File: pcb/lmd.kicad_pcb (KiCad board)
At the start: 2 copper layers, 22.6 x 26.5 mm, 27 parts, among them J1 Conn_01x05, J2 conn:Conn_01x04, J3 Conn_01x03, J4 Conn_01x04, J6 conn:Conn_01x04, U1 TLE493D, U2 TJA1028, U3 DRV8848, U4 PIC16(L)F15323

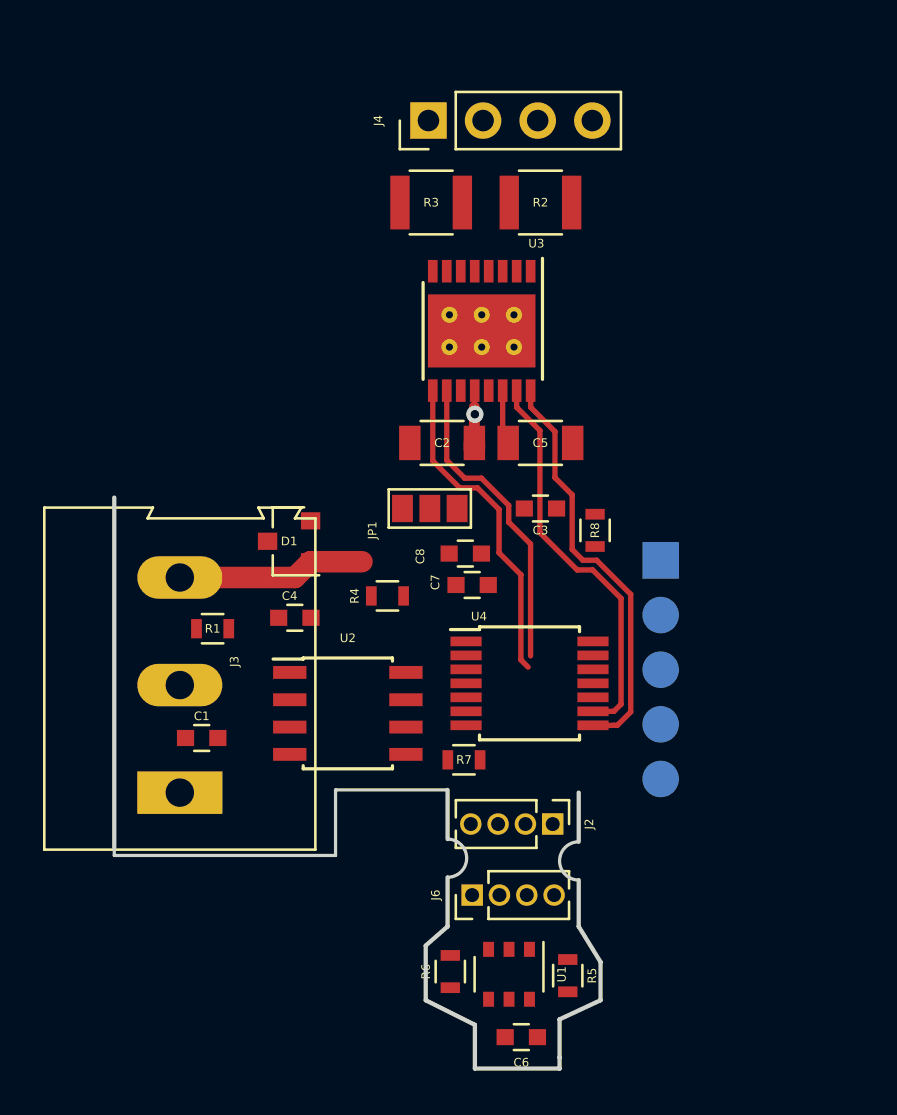
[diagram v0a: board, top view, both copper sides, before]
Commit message: Layout fix
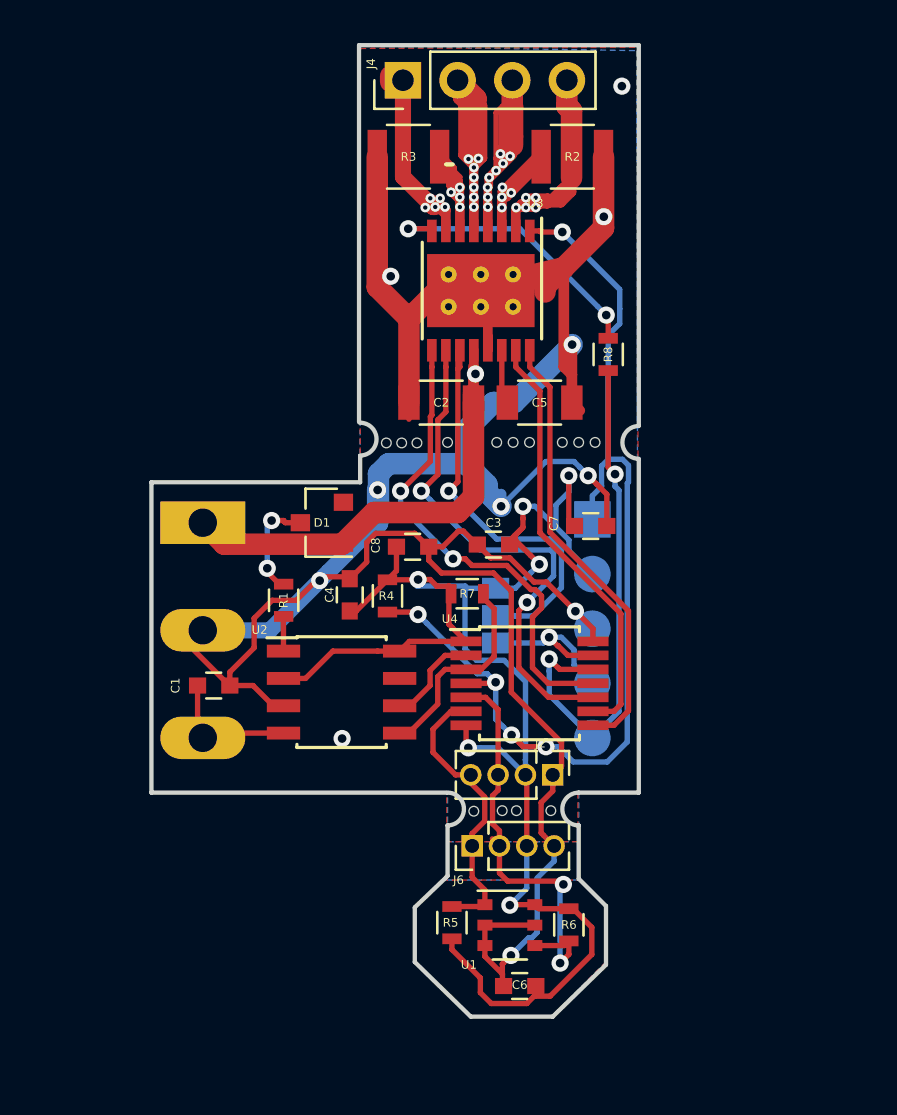
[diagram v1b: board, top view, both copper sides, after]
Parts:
- removed the J6 at (120.8, 129.2)
- added J6: Conn_01x04, ucan_custom:hole, F.Cu at (117.5, 108.2)
- added J6: Conn_01x04, ucan_custom:hole, F.Cu at (116.8, 108.2)
- added J6: Conn_01x04, ucan_custom:hole, F.Cu at (124.4, 125.3)
- added J6: Conn_01x04, ucan_custom:hole, F.Cu at (120.9, 125.3)
- added J6: Conn_01x04, ucan_custom:hole, F.Cu at (122.2, 125.3)
- added J6: Conn_01x04, ucan_custom:hole, F.Cu at (122.8, 125.3)
- added J6: Conn_01x04, Pin_Headers:Pin_Header_Straight_1x04_Pitch1.27mm, F.Cu at (120.8, 126.9)
- added J6: Conn_01x04, ucan_custom:hole, F.Cu at (126.5, 108.2)
- added J6: Conn_01x04, ucan_custom:hole, F.Cu at (125.7, 108.2)
- added J6: Conn_01x04, ucan_custom:hole, F.Cu at (125.0, 108.2)
- added J6: Conn_01x04, ucan_custom:hole, F.Cu at (123.4, 108.2)
- added J6: Conn_01x04, ucan_custom:hole, F.Cu at (122.7, 108.2)
- added J6: Conn_01x04, ucan_custom:hole, F.Cu at (121.9, 108.2)
- added J6: Conn_01x04, ucan_custom:hole, F.Cu at (119.6, 108.2)
- added J6: Conn_01x04, ucan_custom:hole, F.Cu at (118.2, 108.2)
- J2: value conn:Conn_01x04 -> Conn_01x04
- J3, JP1: moved to B.Cu
- U1: value TLE493D -> TLE493D/TLV493
- U4: value PIC16(L)F15323 -> PIC16(L)F15323/PIC16(L)F15325
- moved J3 12.6 mm to (108.3, 111.9), turned to 270 degrees
- moved R8 8.20 mm to (127.1, 104.1)
- moved R7 7.72 mm to (120.5, 115.2), turned to 180 degrees
- moved C7 6.16 mm to (126.3, 112.1)
- moved R6 5.92 mm to (125.3, 130.6)
- moved R5 5.92 mm to (119.8, 130.5)
- moved JP1 5.84 mm to (121.9, 116.2), turned to 180 degrees
- moved J1 3.70 mm to (126.4, 111.8)
- moved R1 3.56 mm to (112.0, 115.5), turned to 90 degrees
- moved C4 2.77 mm to (115.1, 115.3), turned to 90 degrees
- moved C3 2.75 mm to (121.8, 112.9), turned to 180 degrees
- moved R2 2.59 mm to (125.4, 94.9)
- moved C1 2.50 mm to (108.8, 119.5), turned to 0 degrees
- moved C8 2.47 mm to (118.0, 113.0)
- moved R3 2.38 mm to (117.8, 94.9)
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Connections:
- net Net-(JP1-Pad2) renamed DRV_PIN_V
- J2 pad 1: I2C_SDA -> GND
- J2 pad 2: I2C_SCL -> +3V3
- J2 pad 3: +3V3 -> I2C_SDA
- J2 pad 4: GND -> I2C_SCL
- J3 pad 1: Net-(C1-Pad1) -> +12P
- J3 pad 3: +12P -> Net-(C1-Pad1)
- U4 pad 2: LIN_RX -> LIN_TX
- U4 pad 3: LIN_TX -> LIN_RX
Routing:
- net GND: track 0.00 -> 146.1 mm, vias 0 -> 11
- net +3V3: track 0.00 -> 77.4 mm, vias 0 -> 6
- net DRV_SLEEP: track 0.00 -> 47.3 mm, vias 0 -> 5
- net Net-(J4-Pad2): track 0.00 -> 26.1 mm, vias 0 -> 7
- net ICSPCLK: track 0.00 -> 24.5 mm, vias 0 -> 2
- net Net-(J4-Pad3): track 0.00 -> 20.7 mm, vias 0 -> 8
- net I2C_SDA: track 0.00 -> 20.7 mm, vias 0 -> 2
- net DRV_PIN_V: track 0.00 -> 19.4 mm, vias 0 -> 1
- net Net-(J4-Pad1): track 0.00 -> 17.6 mm, vias 0 -> 5
- net Net-(J4-Pad4): track 0.00 -> 14.7 mm, vias 0 -> 5
- net I2C_SCL: track 0.00 -> 13.5 mm
- net DRV_FAULT: track 0.00 -> 13.1 mm, vias 0 -> 2
- net +12P: track 11.5 -> 22.5 mm
- net /DRV_B2: track 14.4 -> 24.4 mm, vias 0 -> 2
- net LIN_RX: track 0.00 -> 9.74 mm
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- added copper zone on B.Cu, net GND
- added copper zone on F.Cu, net GND
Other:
- board size 22.6 x 26.5 mm -> 22.7 x 45.2 mm
- net class Default: clearance 0.2 -> 0.1
- rule trace_clearance: 0.2 -> 0.1
- board text added: "12V"
- board text added: "3V3"
- board text added: "3v3"
- board text added: "A1"
- board text added: "A2"
- board text added: "B1"
- board text added: "B2"
- board text added: "CAN"
- board text added: "CLK"
- board text added: "DAT"
- board text added: "DCMD1.0"
- board text added: "GND"
- board text added: "LIN"
- board text added: "MCLR"
- board text added: "SCL"
- board text added: "SDA"
- board text added: "U"

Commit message: DRV use
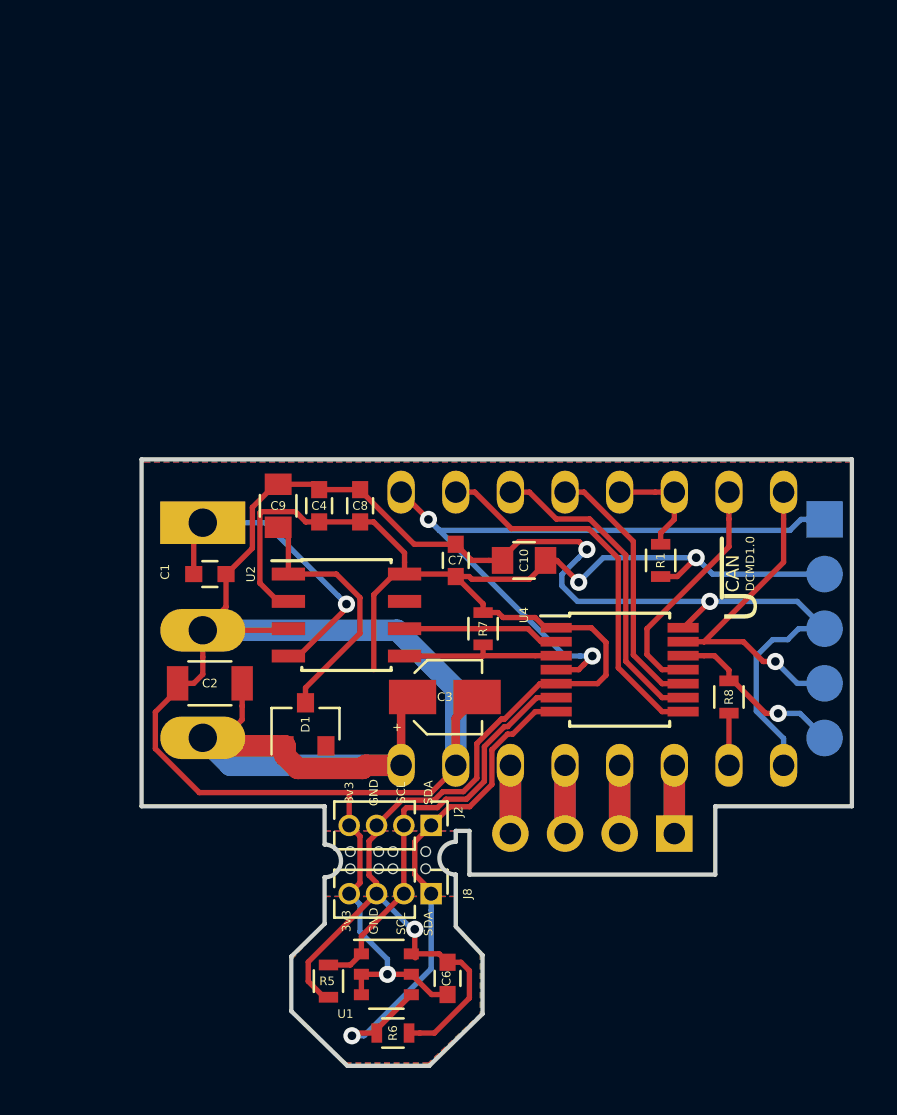
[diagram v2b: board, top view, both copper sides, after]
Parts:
- removed C5: 2.2U, Capacitors_SMD:C_1206
- removed J4: Conn_01x04, Pin_Headers:Pin_Header_Straight_1x04_Pitch2.54mm
- removed the J6 at (117.5, 108.2)
- removed the J6 at (116.8, 108.2)
- removed the J6 at (120.8, 126.9)
- removed the J6 at (126.5, 108.2)
- removed the J6 at (125.7, 108.2)
- removed the J6 at (125.0, 108.2)
- removed the J6 at (123.4, 108.2)
- removed the J6 at (122.7, 108.2)
- removed the J6 at (121.9, 108.2)
- removed the J6 at (119.6, 108.2)
- removed the J6 at (118.2, 108.2)
- removed JP1: Jumper_NC_Dual, Connectors:GS3
- removed R2, R3: 0, Resistors_SMD:R_1210
- removed R4: 10k, Resistors_SMD:R_0603
- added C10: 4,7u, Capacitors_SMD:C_0805, F.Cu at (123.2, 113.7)
- added C9: 4,7u, Capacitors_SMD:C_0805, F.Cu at (111.8, 111.1)
- added J6: Conn_01x04, ucan_custom:hole, F.Cu at (118.6, 128.0)
- added J6: Conn_01x04, ucan_custom:hole, F.Cu at (117.1, 128.0)
- added J6: Conn_01x04, ucan_custom:hole, F.Cu at (116.4, 128.0)
- added J6: Conn_01x04, ucan_custom:hole, F.Cu at (115.1, 128.0)
- added J8: Conn_01x04, Pin_Headers:Pin_Header_Straight_1x04_Pitch1.27mm, F.Cu at (118.9, 129.2)
- added P1: CONN_01X04, Pin_Headers:Pin_Header_Straight_1x04_Pitch2.54mm, B.Cu at (130.2, 126.4)
- C3: value 0.1u -> 10u; footprint Capacitors_SMD:C_0603 -> Capacitors_SMD:CP_Elec_3x5.3
- R1: value 50 -> 10k
- U3: value DRV8848 -> POLOLU_DRV8825/DRV8801; footprint Housings_SSOP:HTSSOP-16-1EP_4.4x5mm_Pitch0.65mm_ThermalVias -> ucan_custom:POLOLU_DRV8825_DRV8801; moved to B.Cu
- moved R1 17.6 mm to (129.5, 113.7)
- moved C2 16.9 mm to (108.6, 119.4)
- moved R8 16.9 mm to (132.7, 120.0), turned to 270 degrees
- moved U3 16.6 mm to (126.4, 116.8), turned to 0 degrees
- moved J1 10.8 mm to (137.2, 111.8)
- moved R6 9.60 mm to (117.1, 135.6), turned to 0 degrees
- moved D1 9.40 mm to (113.0, 121.3), turned to 90 degrees
- moved C3 7.44 mm to (119.5, 120.0), turned to 0 degrees
- moved C7 6.47 mm to (120.0, 113.7), turned to 90 degrees
- moved R5 6.35 mm to (114.1, 133.2)
- moved U1 6.18 mm to (116.8, 132.9)
- moved J6 6.14 mm to (118.6, 127.3)
- moved J2 6.12 mm to (118.9, 126.0)
- moved J6 6.06 mm to (115.1, 127.3)
- moved J6 6.05 mm to (116.4, 127.2)
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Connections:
- net DRV_SLEEP renamed DRV_nENABLE
- C3 pad 1: +3V3 -> +12P
- D1 pad 1: Net-(D1-Pad1) -> Net-(C9-Pad2)
- J1 pad 4: DRV_VREF -> DRV_DIR
- J2 pad 1: GND -> I2C_SDA
- J2 pad 2: +3V3 -> I2C_SCL
- J2 pad 3: I2C_SDA -> +3V3
- J2 pad 4: I2C_SCL -> GND
- J3 pad 1: +12P -> Net-(C1-Pad1)
- J3 pad 3: Net-(C1-Pad1) -> +12P
- R1 pad 1: Net-(R1-Pad1) -> +3V3
- R1 pad 2: Net-(D1-Pad1) -> Net-(R1-Pad2)
- R8 pad 2: DRV_FAULT -> DRV_nFAULT
- U2 pad 1: Net-(R1-Pad1) -> Net-(C9-Pad2)
- U3 pad 10: /DRV_B2 -> DRV_nFAULT
- U3 pad 11: DRV_PIN_V -> Net-(P1-Pad1)
- U3 pad 12: +12P -> Net-(P1-Pad2)
- U3 pad 13: GND -> Net-(P1-Pad3)
- U3 pad 15: /DRV_A2 -> GND
- U3 pad 16: /DRV_A1 -> +12P
- U3 pad 2: Net-(J4-Pad4) -> DRV_MS1
- U3 pad 3: Net-(R2-Pad2) -> DRV_MS2
- U3 pad 4: Net-(J4-Pad3) -> DRV_MS3
- U3 pad 5: Net-(J4-Pad2) -> Net-(R1-Pad2)
- U3 pad 6: Net-(R3-Pad2) -> Net-(R1-Pad2)
- U3 pad 7: Net-(J4-Pad1) -> DRV_STEP
- U3 pad 8: DRV_FAULT -> DRV_DIR
- U3 pad 9: /DRV_B1 -> GND
- U4 pad 10: /DRV_B2 -> DRV_MS3
- U4 pad 11: /DRV_B1 -> DRV_STEP
- U4 pad 13: DRV_VREF -> DRV_DIR
- U4 pad 5: I2C_SDA -> +3V3
- U4 pad 7: +3V3 -> I2C_SDA
- U4 pad 8: /DRV_A1 -> DRV_MS1
- U4 pad 9: /DRV_A2 -> DRV_MS2
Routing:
- net GND: track 146.1 -> 112.6 mm, vias 11 -> 3
- net Net-(J4-Pad2): track 26.1 -> 0.00 mm, vias 7 -> 0
- net /DRV_B2: track 24.4 -> 0.00 mm, vias 2 -> 0
- net /DRV_B1: track 22.8 -> 0.00 mm, vias 2 -> 0
- net Net-(J4-Pad3): track 20.7 -> 0.00 mm, vias 8 -> 0
- net /DRV_A1: track 20.6 -> 0.00 mm
- net /DRV_A2: track 19.9 -> 0.00 mm
- net DRV_PIN_V: track 19.4 -> 0.00 mm, vias 1 -> 0
- net DRV_MS1: track 0.00 -> 17.8 mm
- net Net-(J4-Pad1): track 17.6 -> 0.00 mm, vias 5 -> 0
- net +12P: track 22.5 -> 38.8 mm, vias 1 -> 0
- net ICSPCLK: track 24.5 -> 8.45 mm, vias 2 -> 1
- net DRV_DIR: track 0.00 -> 15.9 mm, vias 0 -> 1
- net DRV_MS2: track 0.00 -> 14.9 mm
- net Net-(J4-Pad4): track 14.7 -> 0.00 mm, vias 5 -> 0
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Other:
- board size 22.7 x 45.2 mm -> 33 x 28.2 mm
- board text removed: "A1"
- board text removed: "A2"
- board text removed: "B1"
- board text removed: "B2"
